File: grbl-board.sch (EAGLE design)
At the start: 32 parts, among them IC1 MEGA8-P, IC2 FT232RL, IC3 ADUM1250, IC4 LM2596S, Q1 16 MHz, X1 PN61729-S, X5 22-23-2021

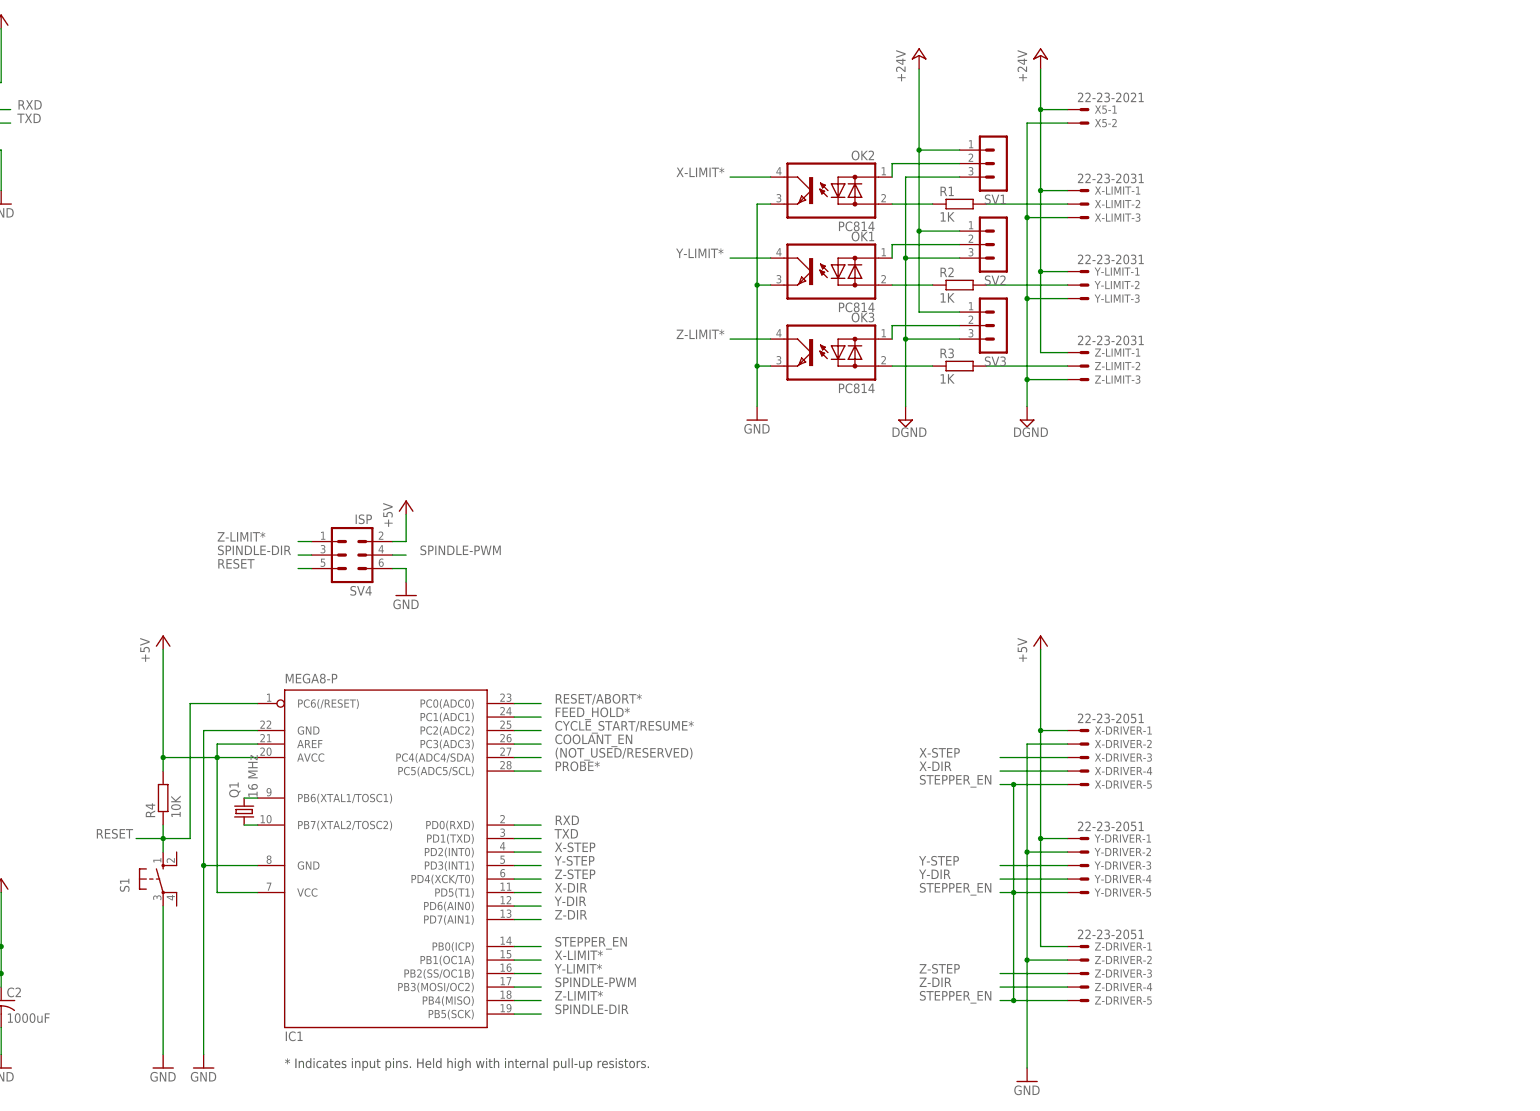
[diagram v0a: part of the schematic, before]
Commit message: add buttons
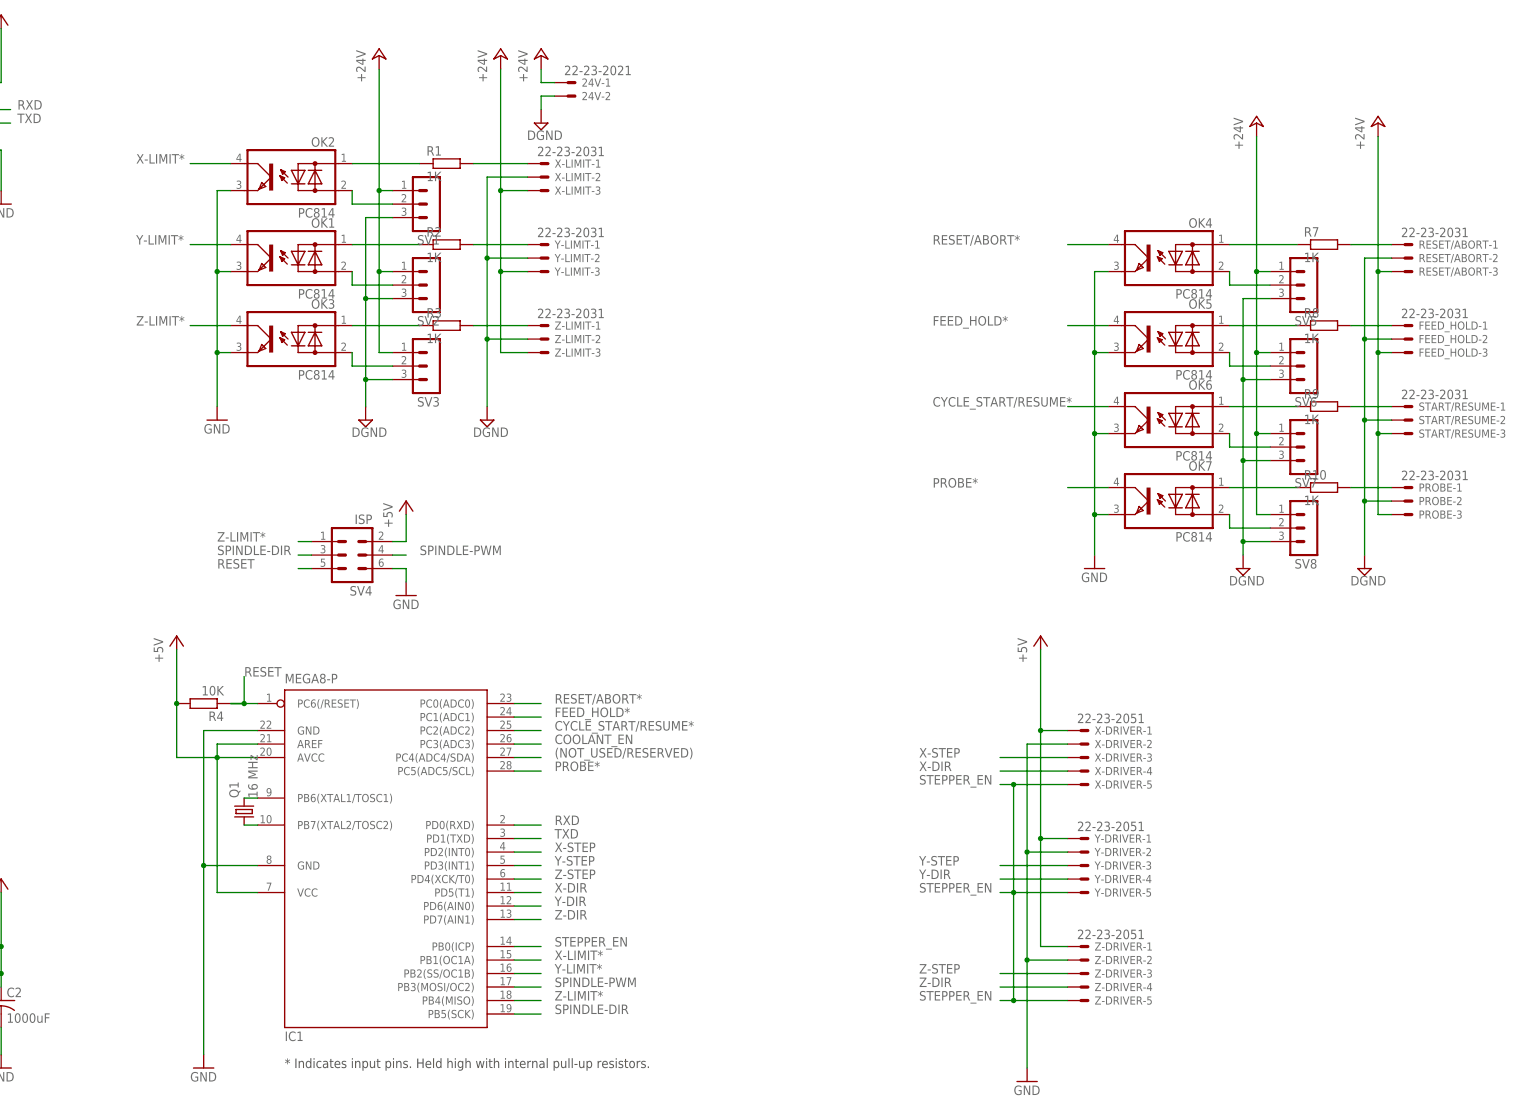
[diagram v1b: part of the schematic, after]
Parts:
- removed S1: (no value), switch-omron:10-XX
- removed X5: 22-23-2021, con-molex:22-23-2021
- added 24V: 22-23-2021, con-molex:22-23-2021
- added FEED_HOLD, PROBE, RESET/ABORT, START/RESUME: 22-23-2031, con-molex:22-23-2031
- added OK4, OK5, OK6, OK7: PC814, optocoupler:PC814
- added R10, R7, R8, R9: 1K, resistor:R-EU_M0805
- added SV5, SV6, SV7, SV8: (no value), con-lstb:MA03-1
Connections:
- removed net VDD1: IC3.VDD1
- new net N$17: OK4.AC2, SV5.2
- new net N$20: OK4.AC1, R7.1
- new net N$21: OK5.AC2, SV6.2
- new net N$22: OK6.AC2, SV7.2
- new net N$23: OK7.AC2, SV8.2
- new net N$24: OK5.AC1, R8.1
- new net N$25: OK6.AC1, R9.1
- new net N$26: OK7.AC1, R10.1
- new net N$27: PROBE-1.S, R10.2
- new net N$28: R9.2, START/RESUME-1.S
- new net N$29: FEED_HOLD-1.S, R8.2
- new net N$30: R7.2, RESET/ABORT-1.S
- net +24V: now also 24V-1.S, FEED_HOLD-3.S, PROBE-3.S, RESET/ABORT-3.S, START/RESUME-3.S, SV5.1, SV6.1, SV7.1, SV8.1, X-LIMIT-3.S, Y-LIMIT-3.S, Z-LIMIT-3.S; no longer X-LIMIT-1.S, X5-1.S, Y-LIMIT-1.S, Z-LIMIT-1.S
- net +5V: now also IC3.VDD1
- net CYCLE_START/RESUME*: now also OK6.C
- net DGND: now also 24V-2.S, FEED_HOLD-2.S, PROBE-2.S, RESET/ABORT-2.S, START/RESUME-2.S, SV5.3, SV6.3, SV7.3, SV8.3, X-LIMIT-2.S, Y-LIMIT-2.S, Z-LIMIT-2.S; no longer X-LIMIT-3.S, X5-2.S, Y-LIMIT-3.S, Z-LIMIT-3.S
- net FEED_HOLD*: now also OK5.C
- net GND: now also OK4.E, OK5.E, OK6.E, OK7.E; no longer S1.P
- net N$10: now also R3.1; no longer SV3.2
- net N$11: now also OK3.AC2, SV3.2; no longer OK1.AC1, SV2.2
- net N$12: now also OK2.AC2; no longer OK2.AC1
- net N$13: now also X-LIMIT-1.S; no longer X-LIMIT-2.S
- net N$14: now also OK1.AC2, SV2.2; no longer OK3.AC2, R3.1
- net N$15: now also OK1.AC1; no longer OK1.AC2
- net N$5: now also OK2.AC1; no longer OK2.AC2
- net N$8: now also Y-LIMIT-1.S; no longer Y-LIMIT-2.S
- net N$9: now also Z-LIMIT-1.S; no longer Z-LIMIT-2.S
- net PROBE*: now also OK7.C
- net RESET: no longer S1.S
- net RESET/ABORT*: now also OK4.C
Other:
- moved on the sheet: OK1, OK2, OK3, R1, R2, R3, R4, SV1, SV2, SV3, X-LIMIT-1, X-LIMIT-2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
